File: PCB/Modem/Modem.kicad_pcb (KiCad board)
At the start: 6 copper layers, 64.6 x 58.9 mm, 212 parts, among them IC10 AT32 433, IC11 EN29F040A, IC12 KM681000BLT-7 (I-Reverse), IC13 EA, IC14 E4, IC15 8206 5877, IC16 E3, IC17 EA, IC18 3L01, IC2 EA, IC3 Line-Module, IC4 E5, IC5 MN195, IC6 54, IC7 EA, IC8 TA31033F, IC9 EA, Q1 CQ, Q2 DA QU, Q3 123, Q4 CQ, Q7 SOT-323_SC-70, Q9 HP, SW2 SW_modem, T1 IsoTransformer

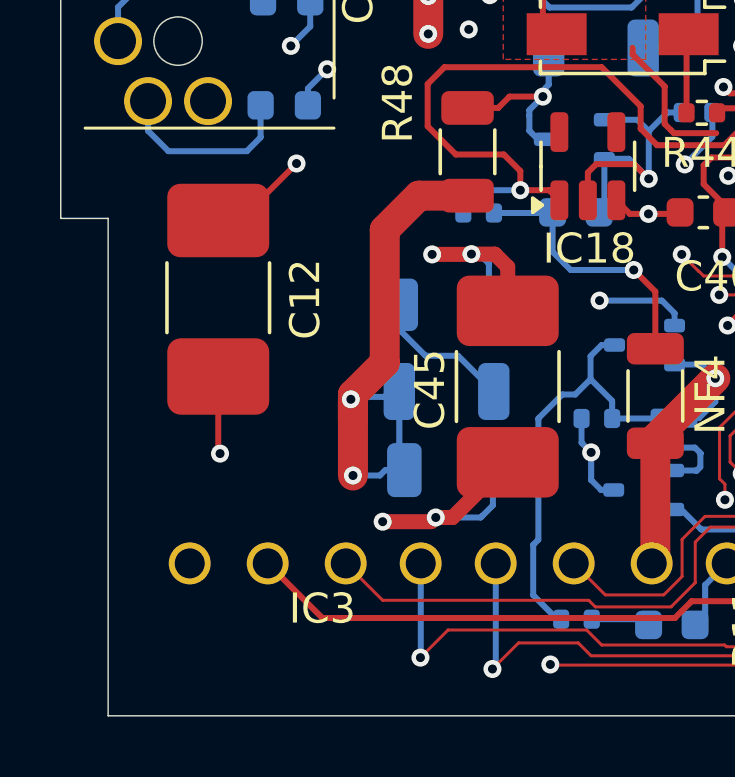
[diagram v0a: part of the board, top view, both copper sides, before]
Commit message: Add files via upload
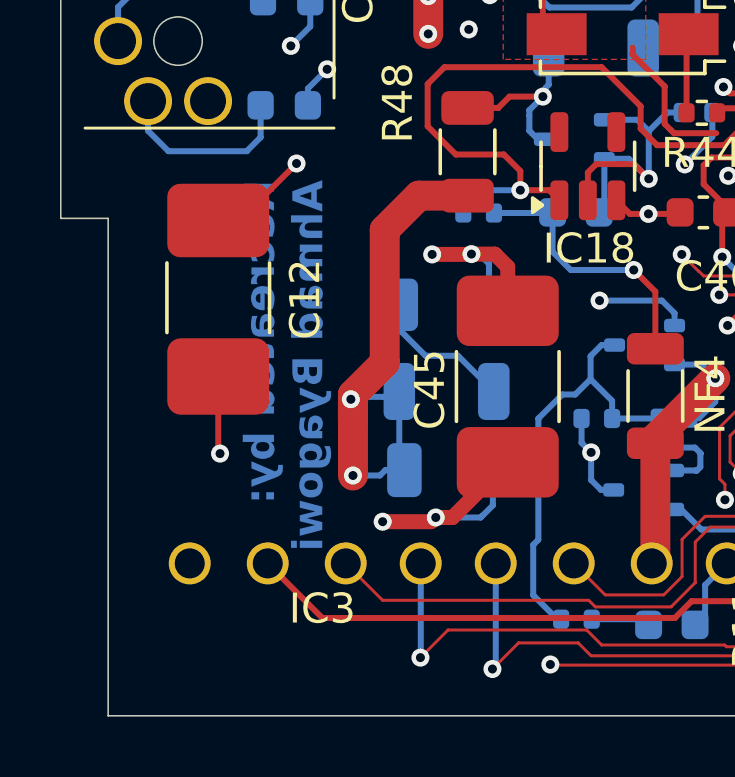
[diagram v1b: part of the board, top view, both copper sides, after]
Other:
- board text added: "Recreated by: Ahmad Byagowi"
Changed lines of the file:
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@@
 		(layer "Edge.Cuts")
+	)
+	(gr_text "Recreated by:\nAhmad Byagowi"
+		(at 127.21 111 90)
+		(layer "B.Cu")
+		(effects
+			(font
+				(size 1 1)
+				(thickness 0.2)
+				(bold yes)
+			)
+			(justify left bottom mirror)
+		)
 	)
 	(segment

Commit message: Add files via upload
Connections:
- net MN195_UC0 renamed MN195_UC1
- IC5 pad 61: MN195_S14 -> MN195_S15
